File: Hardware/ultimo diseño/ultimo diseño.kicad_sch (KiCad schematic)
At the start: 33 parts, among them J1 Screw_Terminal_01x02, J2 Screw_Terminal_01x02, J3 Screw_Terminal_01x02, J4 Screw_Terminal_01x02, J5 12V EN SERIE, J6 Screw_Terminal_01x02, SW1 SW_DPST_x2, SW2 SW_DPST_x2, SW3 SW_DPST_x2, U1 AMS1117-3.3, U2 VTB6612_BREAKOUT, U3 AMS1117-5.0, U4 ESP32-S3-WROOM-1-N8

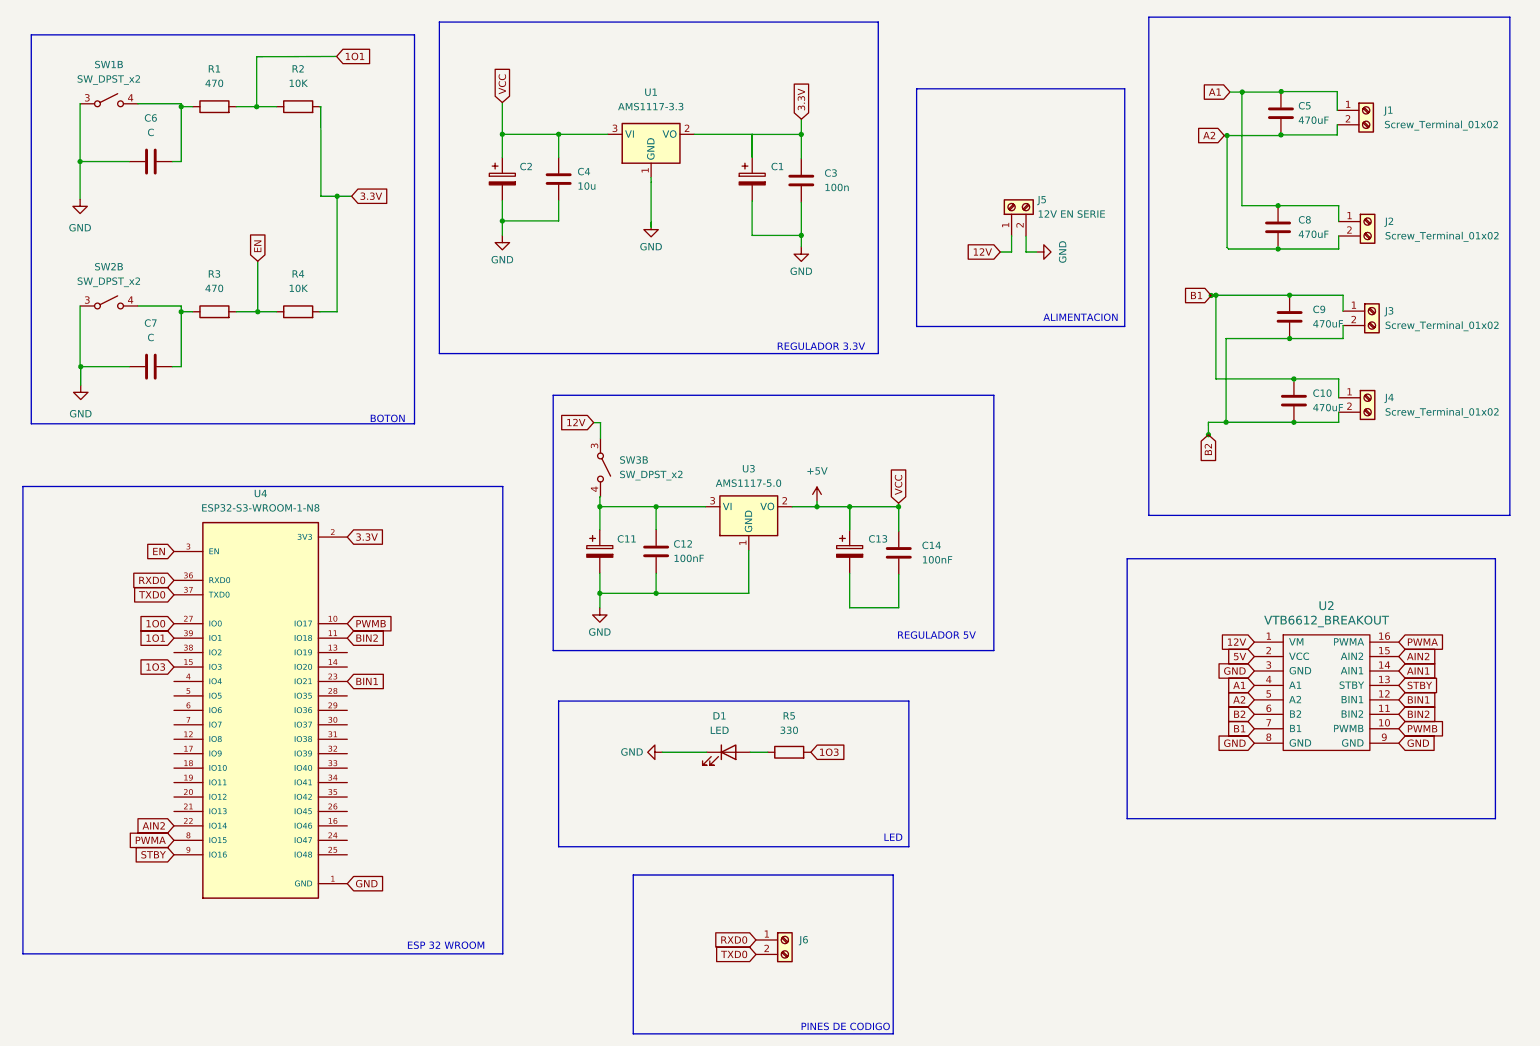
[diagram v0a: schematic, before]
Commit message: 25/5
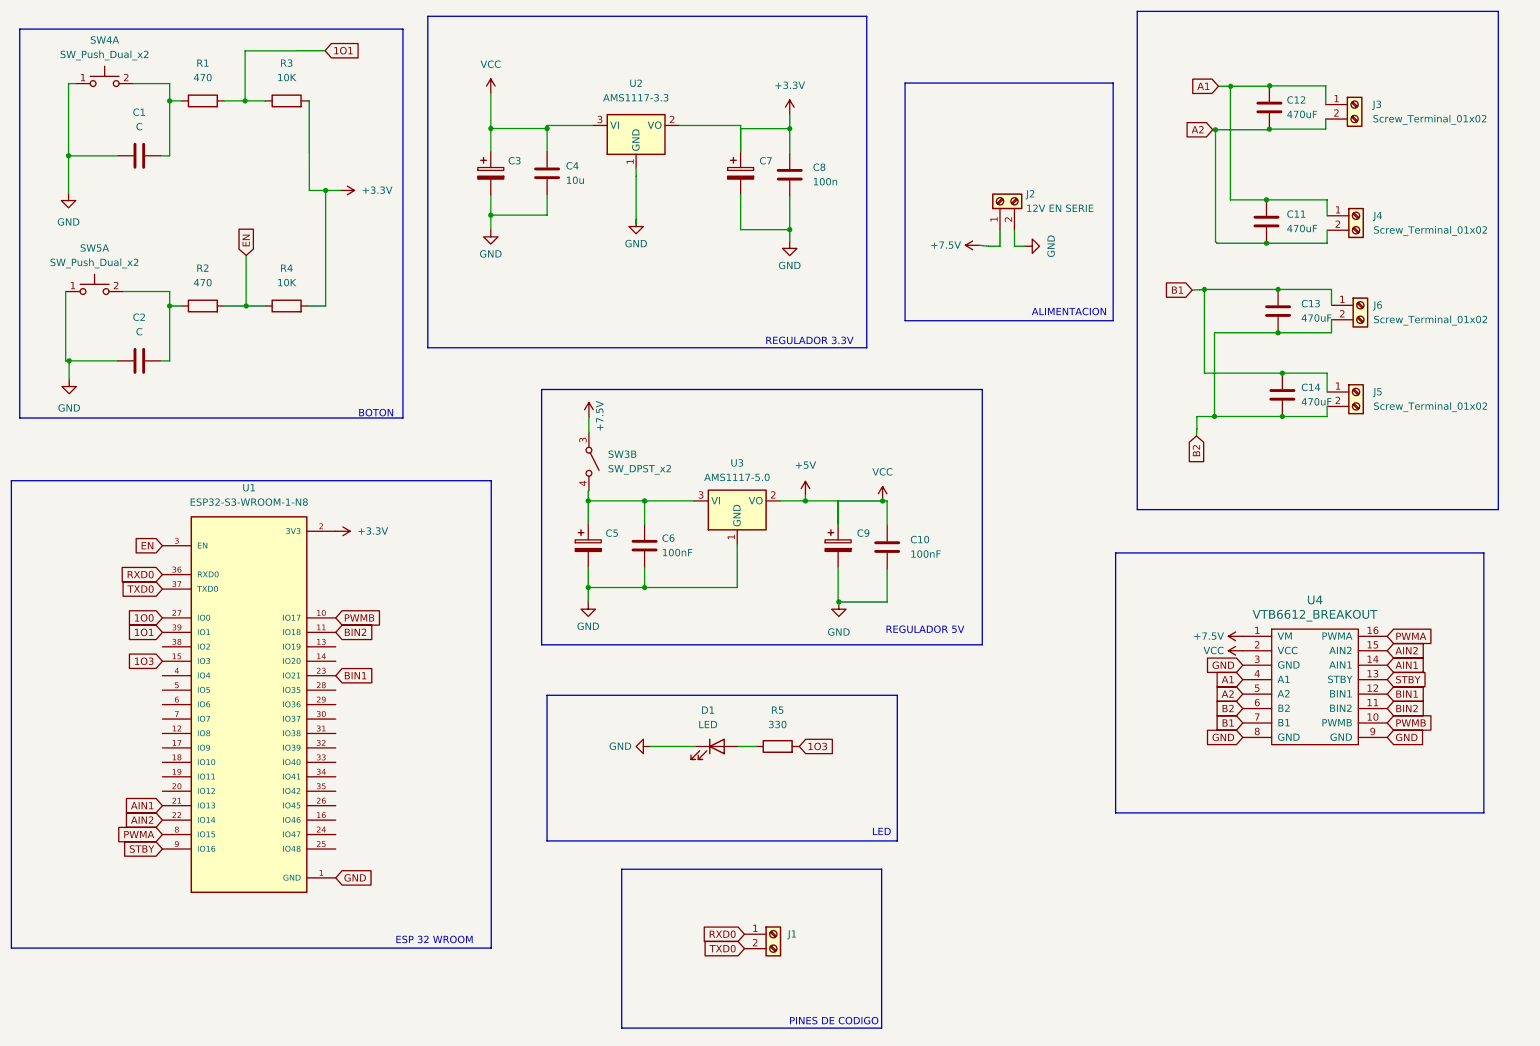
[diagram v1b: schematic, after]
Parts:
- removed C1, C2: 100n, Capacitor_SMD:C_0805_2012Metric, symbol Device:C_Polarized
- removed C11, C13: 100u, Capacitor_SMD:C_0805_2012Metric, symbol Device:C_Polarized
- removed C3: 100n, Capacitor_SMD:C_0805_2012Metric, symbol Device:C
- removed C5, C9: 470uF, Capacitor_THT:C_Disc_D3.0mm_W1.6mm_P2.50mm, symbol Device:C
- removed C7: C, Capacitor_SMD:C_0805_2012Metric, symbol Device:C
- removed SW1, SW2: SW_DPST_x2, Button_Switch_SMD:SW_Push_SPST_NO_Alps_SKRK, symbol Switch:SW_DPST_x2
- removed U1: AMS1117-3.3, Package_TO_SOT_SMD:SOT-223-3_TabPin2, symbol Regulator_Linear:AMS1117-3.3
- removed U2: VTB6612_BREAKOUT, aaa:MODULE_ROB-14450, symbol EESTN5:TB6612_BREAKOUT
- removed U4: ESP32-S3-WROOM-1-N8, ESP32-S3-WROOM-1-N8:XCVR_ESP32-S3-WROOM-1-N8, symbol ian:ESP32-S3-WROOM-1-N8
- added C1, C2: C, Capacitor_SMD:C_0805_2012Metric, symbol Device:C
- added C11, C13: 470uF, Capacitor_THT:C_Disc_D3.0mm_W1.6mm_P2.50mm, symbol Device:C
- added C3, C7: 100n, Capacitor_SMD:C_0805_2012Metric, symbol Device:C_Polarized
- added C5, C9: 100u, Capacitor_SMD:C_0805_2012Metric, symbol Device:C_Polarized
- added SW4, SW5: SW_Push_Dual_x2, Button_Switch_SMD:SW_SPST_B3U-1000P, symbol Switch:SW_Push_Dual_x2
- added U1: ESP32-S3-WROOM-1-N8, ESP32-S3-WROOM-1-N8:XCVR_ESP32-S3-WROOM-1-N8, symbol ian:ESP32-S3-WROOM-1-N8
- added U2: AMS1117-3.3, Package_TO_SOT_SMD:SOT-223-3_TabPin2, symbol Regulator_Linear:AMS1117-3.3
- added U4: VTB6612_BREAKOUT, EESTN5:TB6612_Breakout, symbol EESTN5:TB6612_BREAKOUT
- C10: value 470uF -> 100nF; footprint Capacitor_THT:C_Disc_D3.0mm_W1.6mm_P2.50mm -> Capacitor_SMD:C_0805_2012Metric
- C12, C14: value 100nF -> 470uF; footprint Capacitor_SMD:C_0805_2012Metric -> Capacitor_THT:C_Disc_D3.0mm_W1.6mm_P2.50mm
- C6: value C -> 100nF
- C8: value 470uF -> 100n; footprint Capacitor_THT:C_Disc_D3.0mm_W1.6mm_P2.50mm -> Capacitor_SMD:C_0805_2012Metric
- J1: footprint TerminalBlock:TerminalBlock_MaiXu_MX126-5.0-02P_1x02_P5.00mm -> Connector_PinHeader_1.00mm:PinHeader_1x02_P1.00mm_Horizontal
- J2: value Screw_Terminal_01x02 -> 12V EN SERIE
- J5: value 12V EN SERIE -> Screw_Terminal_01x02
- J6: footprint Connector_PinHeader_1.00mm:PinHeader_1x02_P1.00mm_Horizontal -> TerminalBlock:TerminalBlock_MaiXu_MX126-5.0-02P_1x02_P5.00mm
- R2: value 10K -> 470
- R3: value 470 -> 10K
- SW3: footprint aaa:swicht de 3 -> Button_Switch_THT:SW_Slide-03_Wuerth-WS-SLTV_10x2.5x6.4_P2.54mm
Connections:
- net +5V: now also C10.1, C3.1, C9.1, U2.3 (VI), U4.2 (VCC); no longer C14.1
- net 1O0: now also U1.27 (IO0)
- net 1O1: now also R3.1, U1.39 (IO1); no longer R2.1
- net 1O3: now also U1.15 (IO3)
- net A1: now also C12.1, J3.1 (Pin_1), J4.1 (Pin_1), C11.1, U4.4 (A1); no longer C8.1, J1.1 (Pin_1), J2.1 (Pin_1)
- net A2: now also C12.2, J3.2 (Pin_2), J4.2 (Pin_2), C11.2, U4.5 (A2); no longer C8.2, J1.2 (Pin_2), J2.2 (Pin_2)
- net AIN1: now also U1.21 (IO13), U4.14 (AIN1)
- net AIN2: now also U1.22 (IO14), U4.15 (AIN2)
- net B1: now also C14.1, J5.1 (Pin_1), J6.1 (Pin_1), C13.1, U4.7 (B1); no longer C10.1, J3.1 (Pin_1), J4.1 (Pin_1)
- net B2: now also C14.2, J5.2 (Pin_2), J6.2 (Pin_2), C13.2, U4.6 (B2); no longer C10.2, J3.2 (Pin_2), J4.2 (Pin_2)
- net BIN1: now also U1.23 (IO21), U4.12 (BIN1)
- net BIN2: now also U1.11 (IO18), U4.11 (BIN2)
- net EN: now also R2.2, U1.3 (EN); no longer R3.2
- net GND: now also C10.2, C6.2, C8.2, J2.2 (Pin_2), C1.1, C2.1, C3.2, C5.2, C7.2, C9.2, SW4.1 (C), SW5.1 (C), U1.1 (GND), U1.40 (GND), U1.41_1 (GND), U1.41_2 (GND), U1.41_3 (GND), U1.41_4 (GND), U1.41_5 (GND), U1.41_6 (GND), U1.41_7 (GND), U1.41_8 (GND), U1.41_9 (GND), U2.1 (GND), U4.3 (GND), U4.8 (GND), U4.9 (GND); no longer C12.2, C6.1, J5.2 (Pin_2)
- net PWMA: now also U1.8 (IO15), U4.16 (PWMA)
- net PWMB: now also U1.10 (IO17), U4.10 (PWMB)
- net RXD0: now also J1.1 (Pin_1), U1.36 (RXD0); no longer J6.1 (Pin_1)
- net STBY: now also U1.9 (IO16), U4.13 (STBY)
- net TXD0: now also J1.2 (Pin_2), U1.37 (TXD0); no longer J6.2 (Pin_2)
- net at R1.1: now also C1.2, SW4.2 (D); no longer C6.2
- net at SW3.4 (B), U3.3 (VI): now also C6.1, C5.1; no longer C12.1
- net 12V renamed +7.5V
- net +7.5V: now also J2.1 (Pin_1), U4.1 (VM); no longer J5.1 (Pin_1)
- net 3.3V renamed +3.3V
- net +3.3V: now also C8.1, R3.2, C7.1, U1.2 (3V3), U2.2 (VO); no longer R2.2
- new net: C2.2, R2.1, SW5.2 (D)
